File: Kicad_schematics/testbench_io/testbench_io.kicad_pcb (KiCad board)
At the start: 2 copper layers, 183 x 130 mm, 73 parts, among them J101 Conn_01x02, J102 Conn_01x02, J103 Conn_01x02, J104 DB37_Female_MountingHoles, J301 Conn_01x12, Q201 2N3904, Q301 IPD50R380CE, Q302 IPD50R380CE, Q303 IPD50R380CE, Q304 IPD50R380CE, Q305 IPD50R380CE, Q306 IPD50R380CE, SW101 SW_SPST, SW102 SW_Push, SW103 SW_Push, SW104 SW_Push, SW105 SW_Push, SW106 SW_SPST, SW107 SW_SPST, SW108 SW_DIP_x08, SW109 SW_SPST, SW110 SW_Push, SW111 SW_SPST, SW112 SW_SPST, SW113 SW_SPST, SW114 SW_DPDT_x2, SW201 SW_DIP_x01, U101 NUCLEO64-F476RG, U102 CJMCU_MCP2551, U201 PCF8574AN

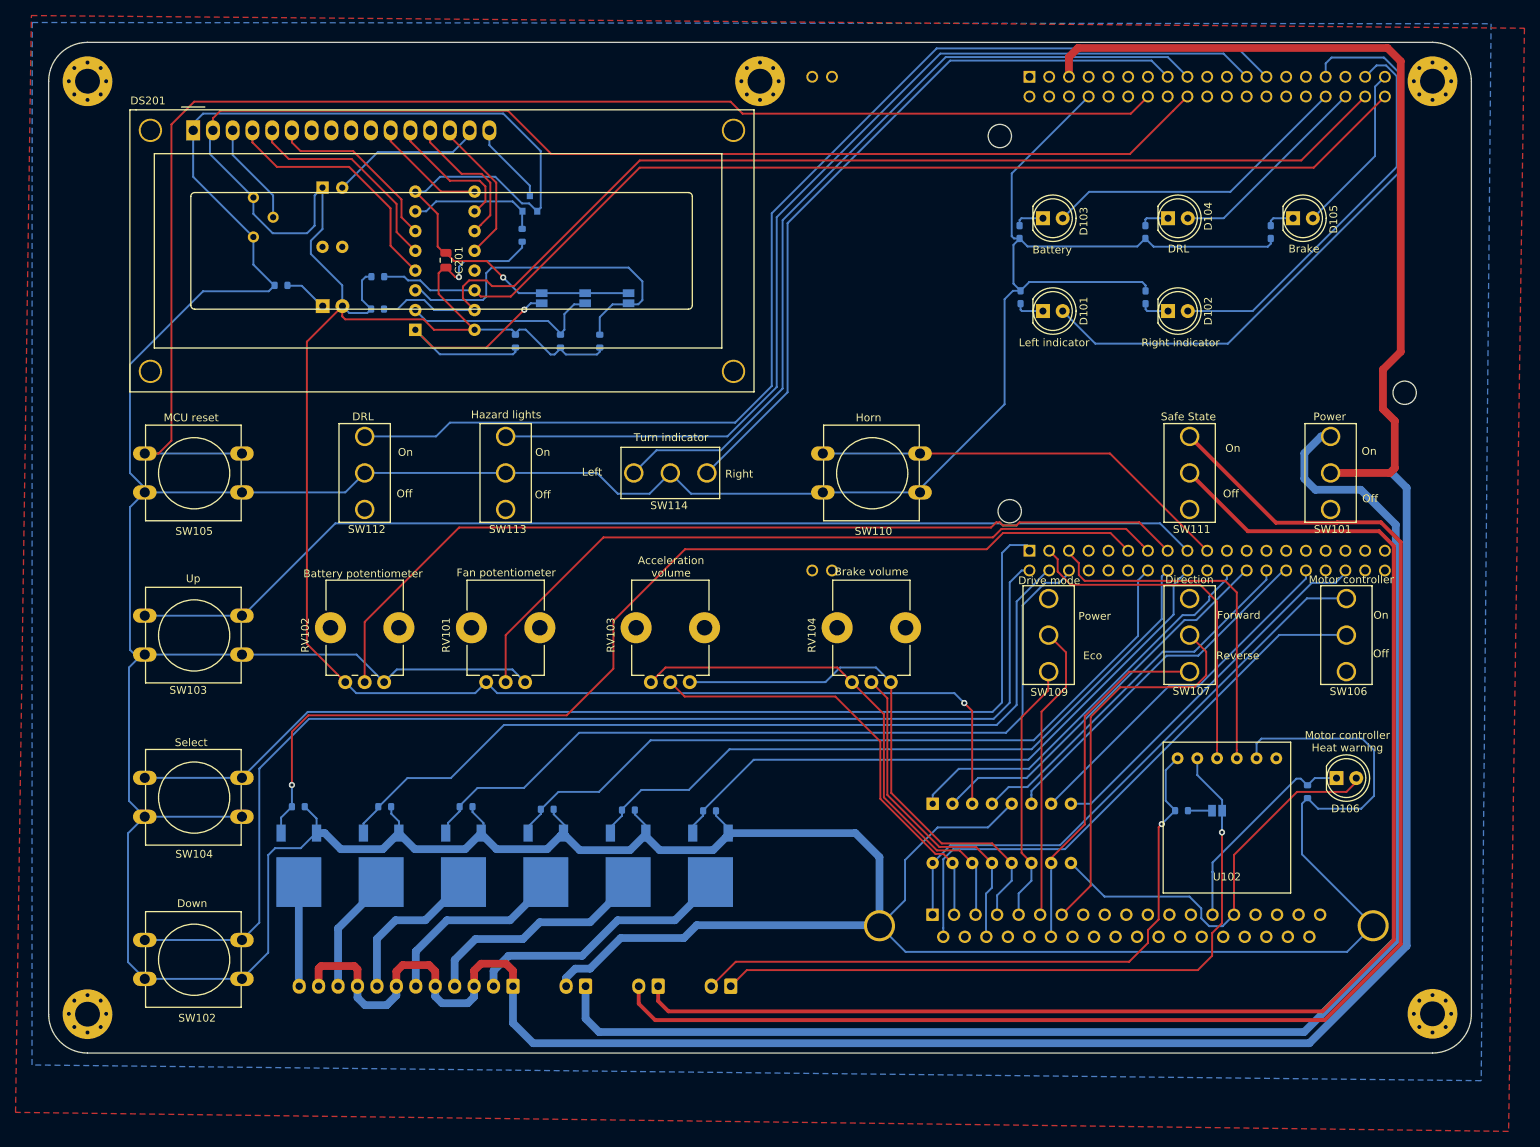
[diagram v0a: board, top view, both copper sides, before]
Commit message: Fixed some final stuff
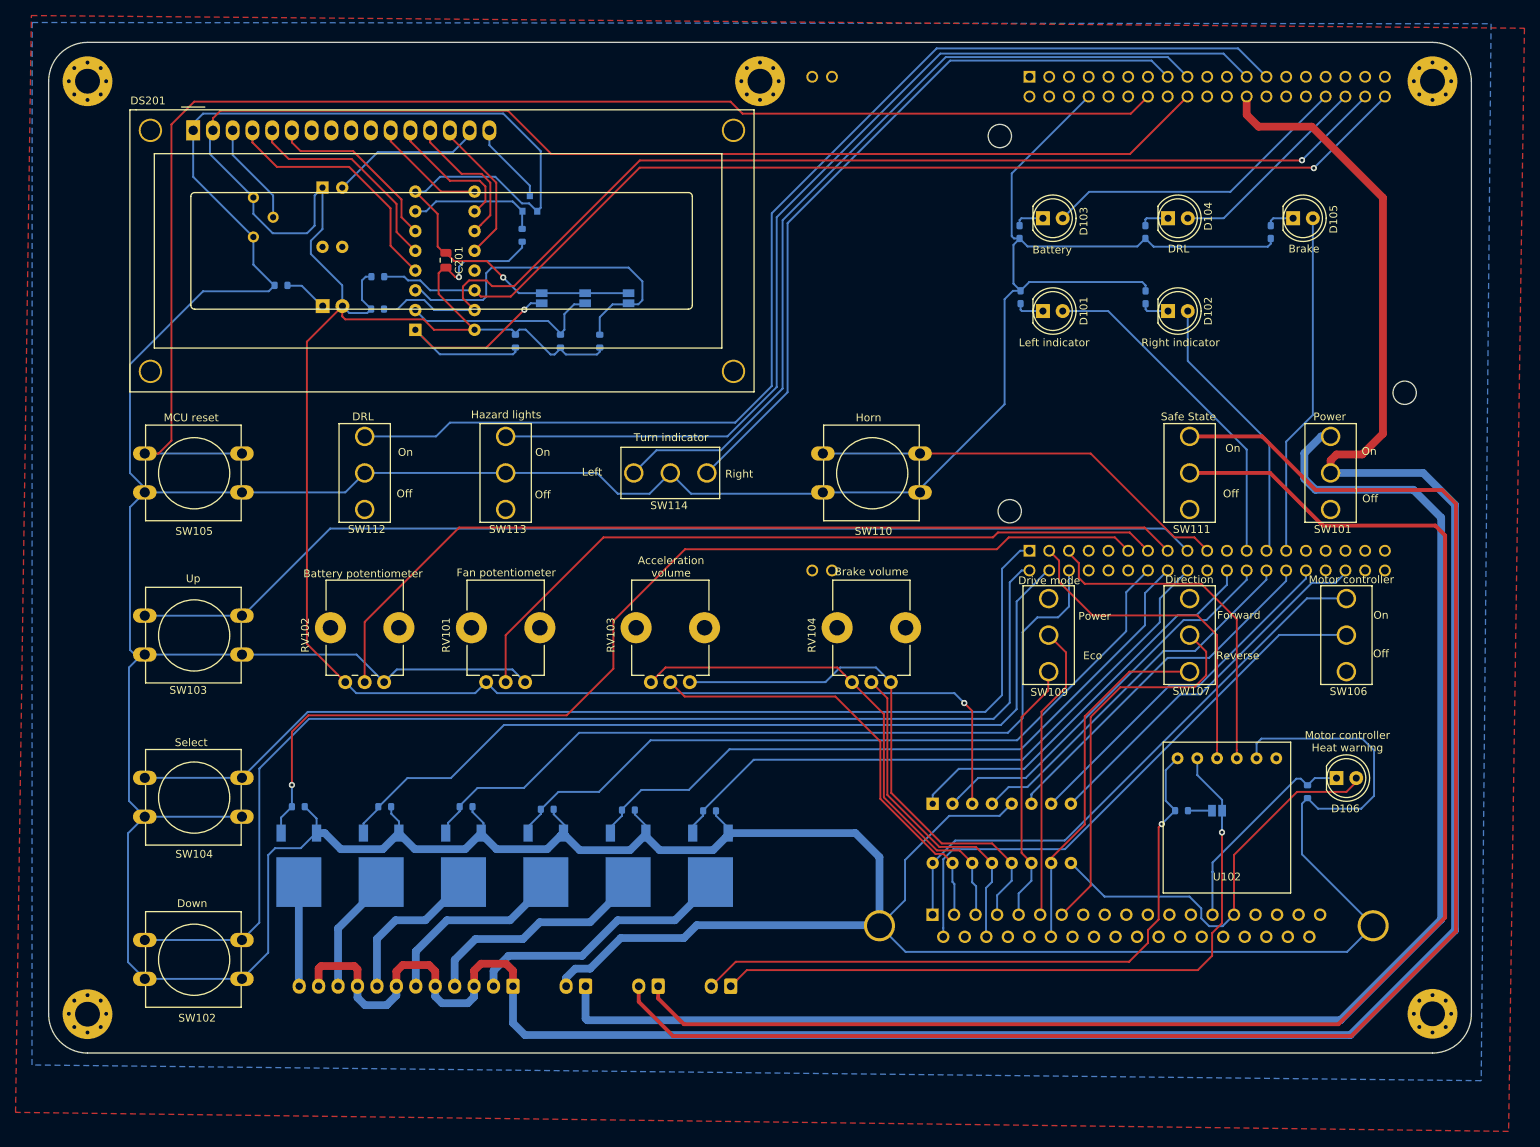
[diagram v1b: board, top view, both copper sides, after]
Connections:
- U101 pad 19: Net-(U101-Pad19) -> GND
- U101 pad 20: Net-(U101-Pad20) -> GND
- U101 pad 22: Net-(U101-Pad22) -> GND
- U101 pad 24: Net-(U101-Pad24) -> VDD_MCU
- U101 pad 31: /Left_LED -> Net-(U101-Pad31)
- U101 pad 35: /Right_LED -> Net-(U101-Pad35)
- U101 pad 37: /Brake_LED -> Net-(U101-Pad37)
- U101 pad 47: Net-(U101-Pad47) -> GND
- U101 pad 5: VDD_MCU -> Net-(U101-Pad5)
- U101 pad 58: Net-(U101-Pad58) -> GND
- U101 pad 61: Net-(U101-Pad61) -> /Left_LED
- U101 pad 63: Net-(U101-Pad63) -> /Right_LED
- U101 pad 65: Net-(U101-Pad65) -> /Brake_LED
- U101 pad 77: Net-(U101-Pad77) -> GND
- U101 pad 78: Net-(U101-Pad78) -> GND
- U101 pad 79: Net-(U101-Pad79) -> GND
- U101 pad 80: Net-(U101-Pad80) -> GND
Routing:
- net /Left_LED: track 79.6 -> 44.1 mm
- net VDD_MCU: track 350.2 -> 314.9 mm
- net /Brake_LED: track 22.0 -> 44.2 mm
- net Net-(J101-Pad2): track 189.7 -> 207.4 mm
- net /Right_LED: track 51.5 -> 35.3 mm
- net Net-(J101-Pad1): track 181.7 -> 195.2 mm
- net V_external: track 189.3 -> 198.7 mm
- net /CRX: track 45.4 -> 43.5 mm
- net /CTX: track 46.2 -> 44.4 mm
- net /Select: track 137.2 -> 135.4 mm
- net /Right_acti: track 99.0 -> 97.8 mm
- net /Battery_pot: track 118.2 -> 117.3 mm
- net /Left_acti: track 90.2 -> 89.4 mm
- net /Up: track 142.0 -> 141.2 mm
- net /Acc_vol: track 50.3 -> 51.0 mm
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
